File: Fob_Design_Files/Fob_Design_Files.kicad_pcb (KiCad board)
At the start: 2 copper layers, 45.6 x 76.8 mm, 34 parts, among them J2 Conn_02x04_Counter_Clockwise, U1 MAX16054AZT_T, U2 CC1101RGPR, U3 BU2032SM-JJ-GTR, U4 STM32C011F4Px, U5 TLV70028_SOT353, Y1 NX3225GA-26.000MHZ-EXS00A-CG0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

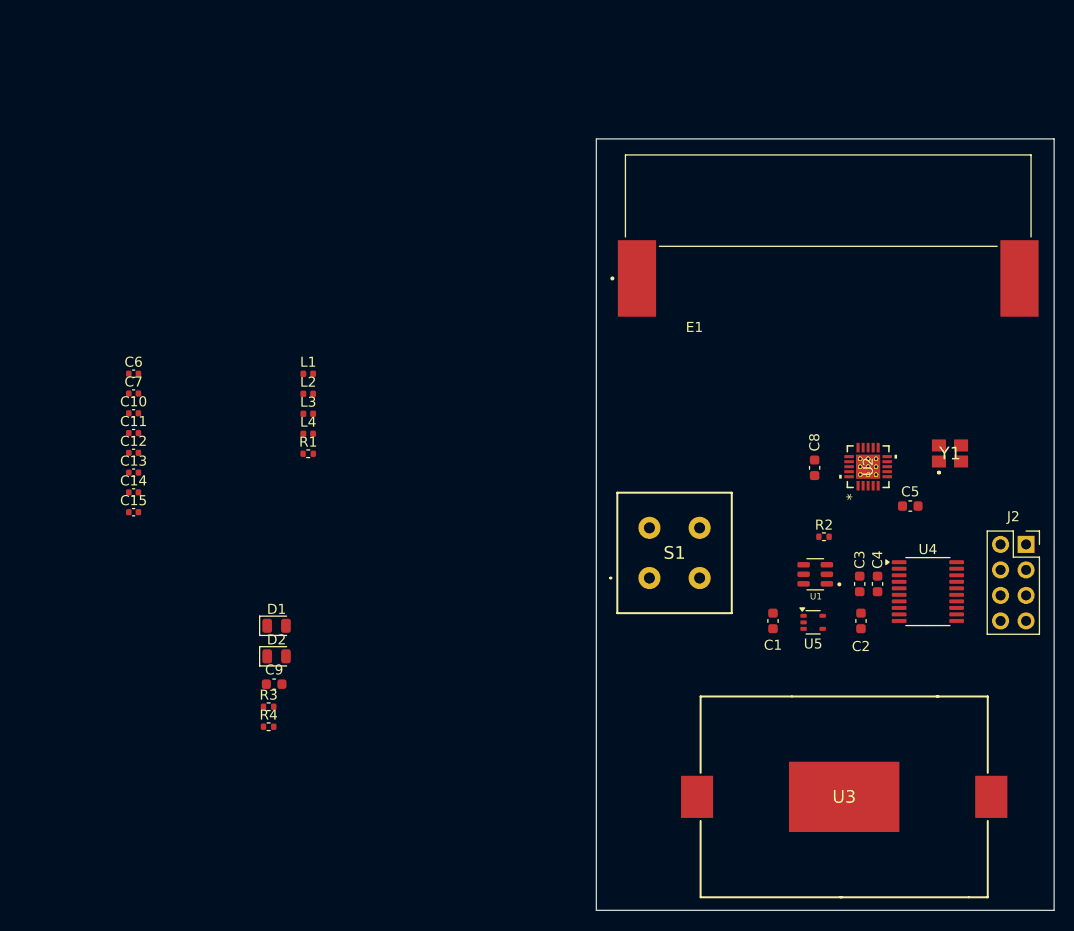
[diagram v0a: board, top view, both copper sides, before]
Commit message: Done with fob layout
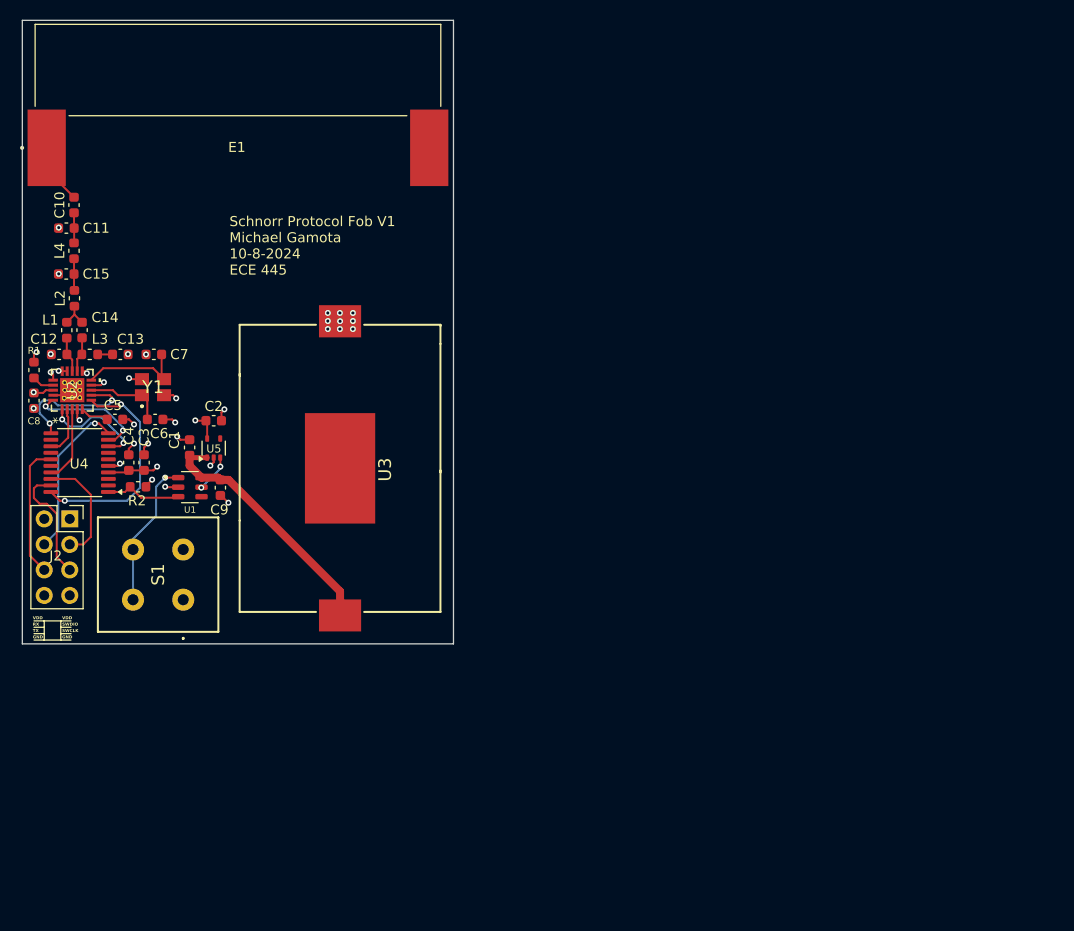
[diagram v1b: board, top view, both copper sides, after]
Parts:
- removed D1, D2: LED, LED_SMD:LED_0805_2012Metric
- removed R3, R4: 330, Resistor_SMD:R_0402_1005Metric
- C10, C11, C12, C13, C14, C15, C6, C7: footprint Capacitor_SMD:C_0402_1005Metric -> Capacitor_SMD:C_0603_1608Metric
- J2: value Conn_02x04_Counter_Clockwise -> Conn_02x04_Odd_Even
- L1, L2, L3, L4: footprint Inductor_SMD:L_0402_1005Metric -> Inductor_SMD:L_0603_1608Metric
- R1, R2: footprint Resistor_SMD:R_0402_1005Metric -> Inductor_SMD:L_0603_1608Metric
- moved J2 95.3 mm to (95.0, 80.0)
- moved U4 85.5 mm to (96.0, 74.4), turned to 180 degrees
- moved C5 79.7 mm to (99.5, 70.1)
- moved Y1 79.7 mm to (103.3, 66.9)
- moved U2 79.6 mm to (95.2, 67.2)
- moved C8 78.0 mm to (91.4, 68.2)
- moved C4 75.6 mm to (100.9, 74.4), turned to 90 degrees
- moved C3 72.3 mm to (102.4, 74.4), turned to 90 degrees
- moved R2 68.5 mm to (101.8, 76.8), turned to 180 degrees
- moved C2 67.5 mm to (109.3, 70.2), turned to 0 degrees
- moved U1 62.9 mm to (107.0, 76.8), turned to 0 degrees
- moved U5 62.2 mm to (109.3, 73.0), turned to 90 degrees
- moved C1 60.6 mm to (106.9, 72.9), turned to 90 degrees
- moved E1 60.2 mm to (111.8, 43.1)
- moved U3 59.9 mm to (121.9, 75.0), turned to 90 degrees
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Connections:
- J2 pad 2: SWDIO -> VDD
- J2 pad 3: SWCLK -> SWDIO
- J2 pad 4: GND -> USART_RX
- J2 pad 5: GND -> SWCLK
- J2 pad 7: USART_RX -> GND
- J2 pad 8: VDD -> GND
- U4 pad 14: RF_RX_LED -> unconnected-(U4-PA7-Pad14)
- U4 pad 16: RF_TX_LED -> unconnected-(U4-PA9/PA11-Pad16)
- U4 pad 17: GDO0 -> GDO2
- U4 pad 20: GDO2 -> GDO0
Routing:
- net VBAT: track 0.00 -> 25.5 mm
- net GDO0: track 0.00 -> 22.2 mm, vias 0 -> 2
- net GND: track 0.00 -> 19.4 mm, vias 0 -> 30
- net USART_RX: track 0.00 -> 16.1 mm, vias 0 -> 1
- net Button: track 0.00 -> 14.8 mm, vias 0 -> 1
- net VDD: track 0.00 -> 14.1 mm, vias 0 -> 7
- net SPI_NSS: track 0.00 -> 13.7 mm, vias 0 -> 2
- net USART_TX: track 0.00 -> 13.3 mm
- net SWCLK: track 0.00 -> 11.8 mm
- net SPI_MOSI: track 0.00 -> 11.8 mm, vias 0 -> 2
- net SWDIO: track 0.00 -> 11.2 mm
- net OSC_OUT: track 0.00 -> 10.8 mm
- net SPI_SCLK: track 0.00 -> 10.7 mm, vias 0 -> 2
- net OSC_IN: track 0.00 -> 7.89 mm
- net PWR_DWN: track 0.00 -> 7.66 mm
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- added copper zone on In1.Cu, net GND
- added copper zone on In2.Cu, net VDD
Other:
- board size 45.6 x 76.8 mm -> 42.9 x 62.1 mm
- copper layers 2 -> 4
- board text added: "GND"
- board text added: "RX"
- board text added: "SWCLK"
- board text added: "SWDIO"
- board text added: "Schnorr Protocol Fob V1 Michael Gamota 10-8-2024 ECE 445"
- board text added: "TX"
- board text added: "VDD"
